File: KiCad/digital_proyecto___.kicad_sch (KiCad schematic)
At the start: 45 parts, among them J10 DE9_Pins, J11 DE9_Pins, U1 74AHCT1G125, U11 MAX3232, U12 A1101xLH, U13 A1101xLH, U2 LM393, U3 LM393, U7 SN65HVD232

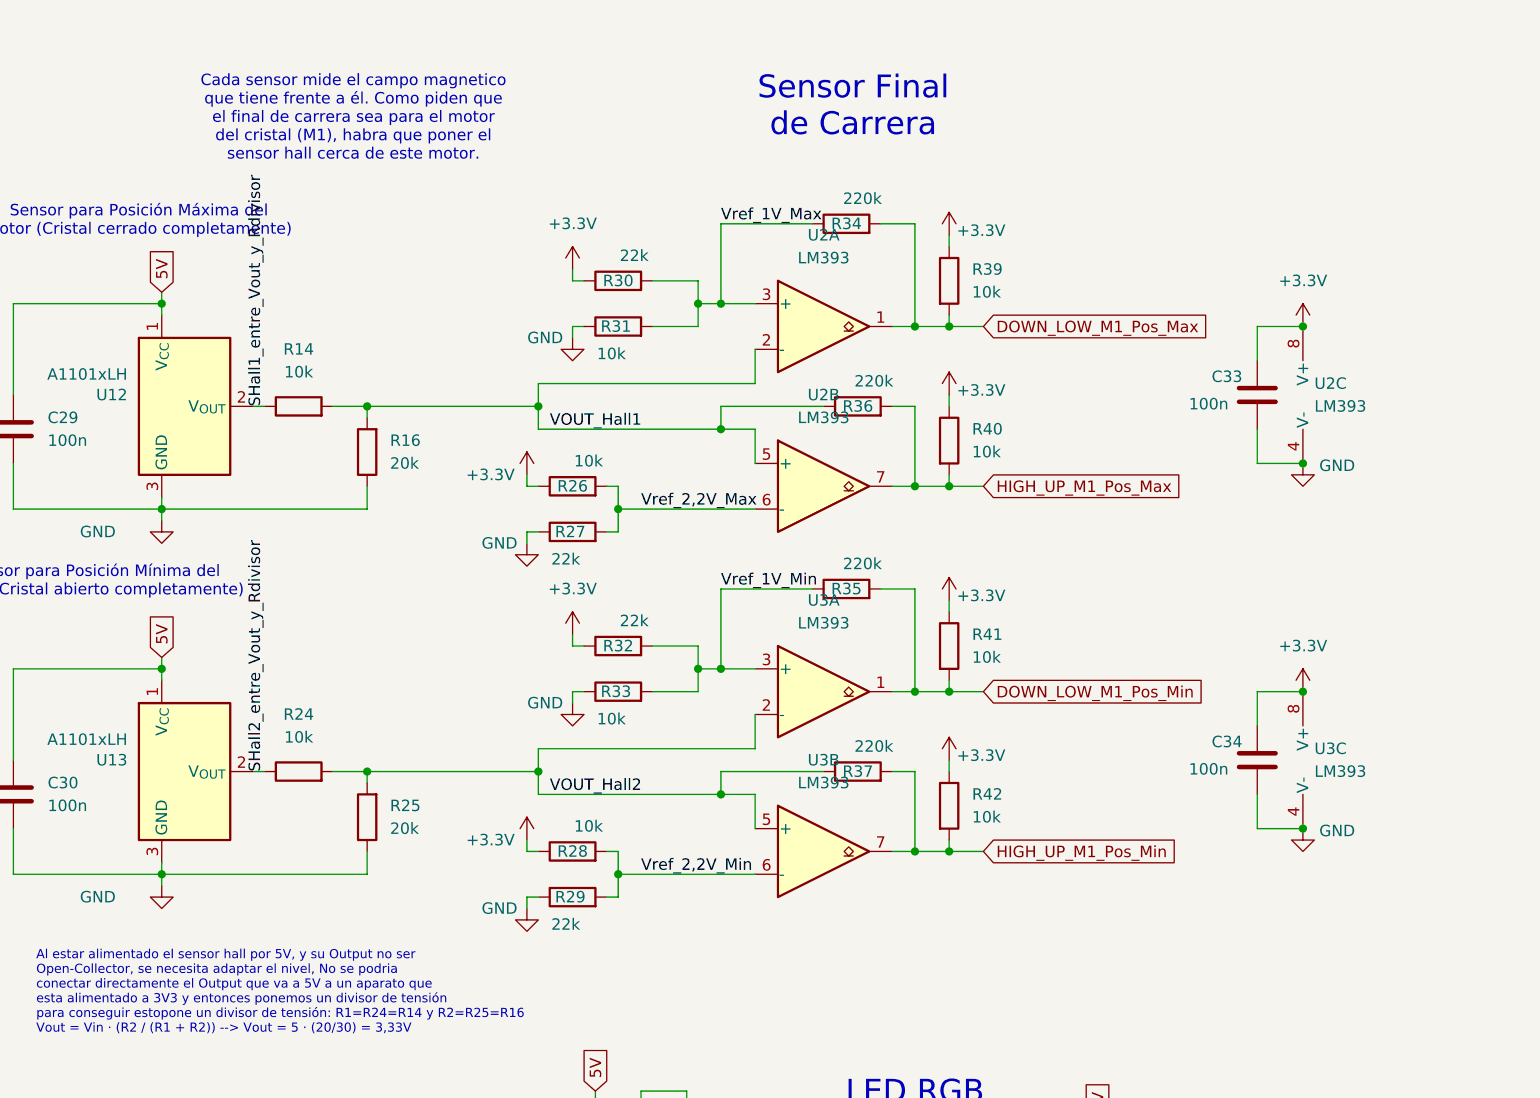
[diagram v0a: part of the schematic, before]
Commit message: Layout definitivo
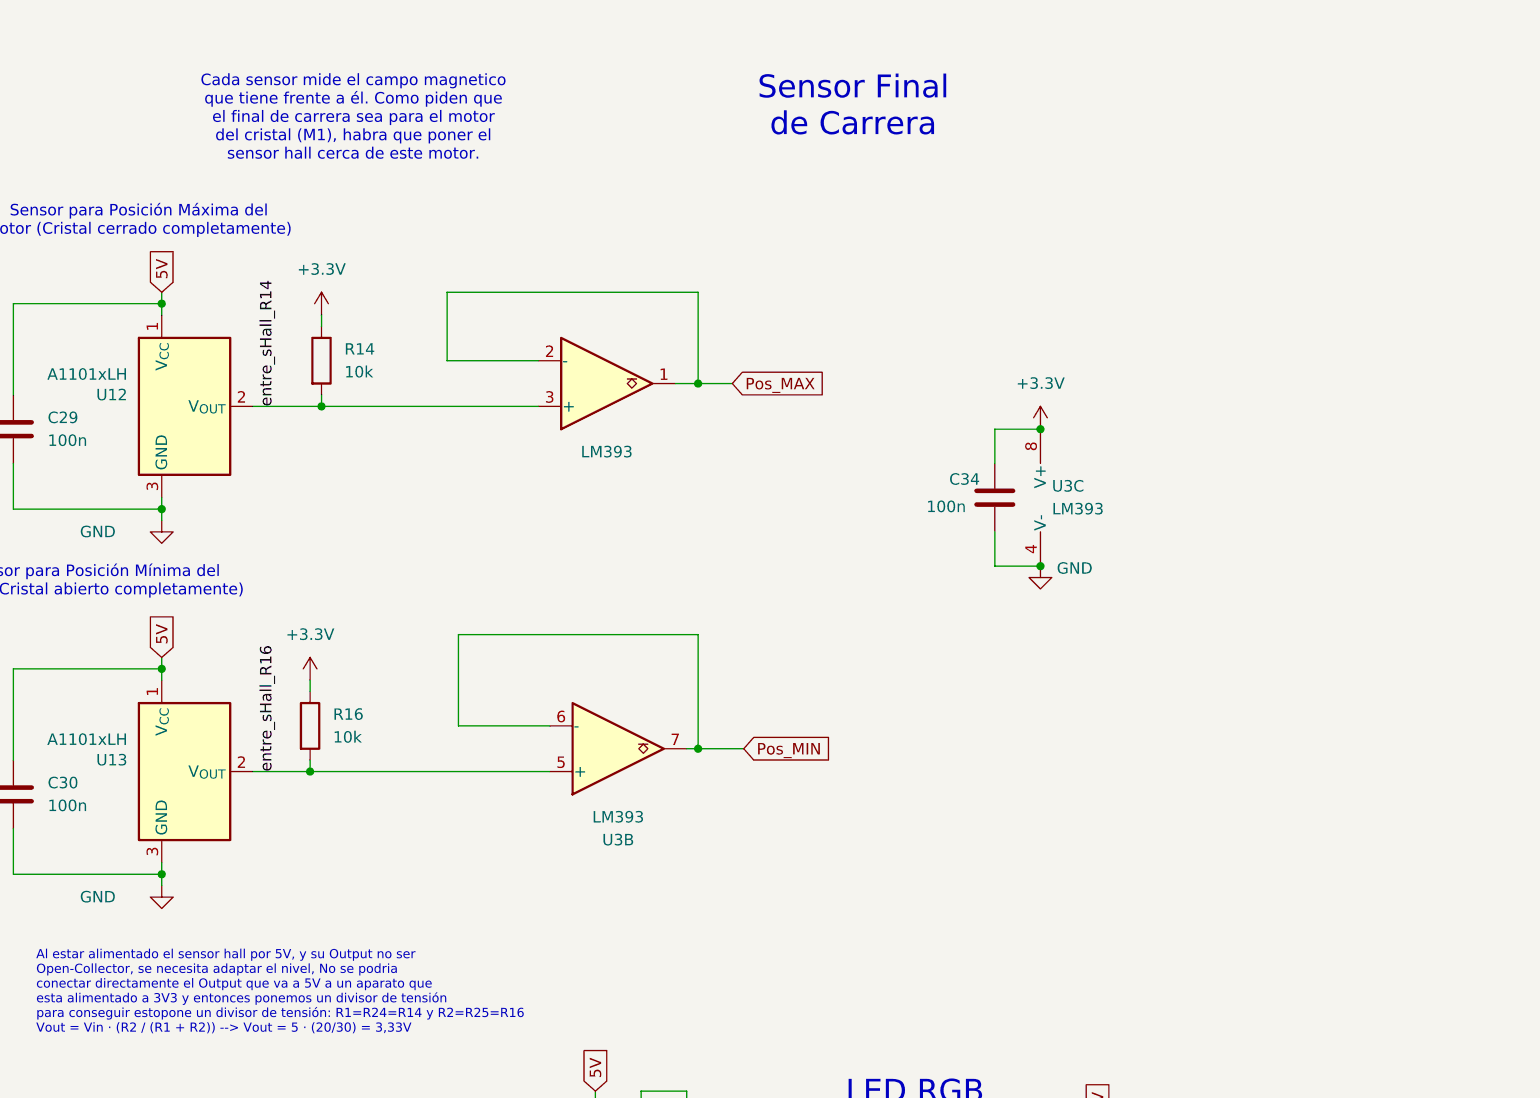
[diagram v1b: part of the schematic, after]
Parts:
- removed C33: 100n, Capacitor_SMD:C_0805_2012Metric, symbol Device:C
- removed R24, R26, R28, R31, R33, R39, R40, R41, R42: 10k, Resistor_SMD:R_0805_2012Metric, symbol Device:R
- removed R25: 20k, Resistor_SMD:R_0805_2012Metric, symbol Device:R
- removed R27, R29, R30, R32: 22k, Resistor_SMD:R_0805_2012Metric, symbol Device:R
- removed R34, R35, R36, R37: 220k, Resistor_SMD:R_0805_2012Metric, symbol Device:R
- removed U2: LM393, Package_SO:SOIC-8_3.9x4.9mm_P1.27mm, symbol Comparator:LM393
- R16: value 20k -> 10k
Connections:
- net Vref_1V_Min is gone; now on net entre_sHall_R14: U3.3 (+)
- net Vref_2,2V_Min is gone; now on net Pos_MIN: U3.6 (-)
- net +3.3V: now also R14.1, R16.1
- net GND: no longer R16.1
- net DOWN_LOW_M1_Pos_Min renamed Pos_MAX
- net Pos_MAX: now also U3.2 (-)
- net HIGH_UP_M1_Pos_Min renamed Pos_MIN
- net SHall1_entre_Vout_y_Rdivisor renamed entre_sHall_R14
- net entre_sHall_R14: now also R14.2; no longer R14.1
- net SHall2_entre_Vout_y_Rdivisor renamed entre_sHall_R16
- net entre_sHall_R16: now also R16.2, U3.5 (+)
- removed net VOUT_Hall1: R14.2, R16.2
- removed net VOUT_Hall2: U3.2 (-), U3.5 (+)
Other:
- moved on the sheet: C34, U3B, U3C
